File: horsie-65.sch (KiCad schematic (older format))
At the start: 17 parts, among them J1 AVR-ISP-6, J2 Connector_Generic_Conn_01x04, SW68 SW_Push, U2 ATmega32U4-AU, Y1 Crystal_GND24_Small

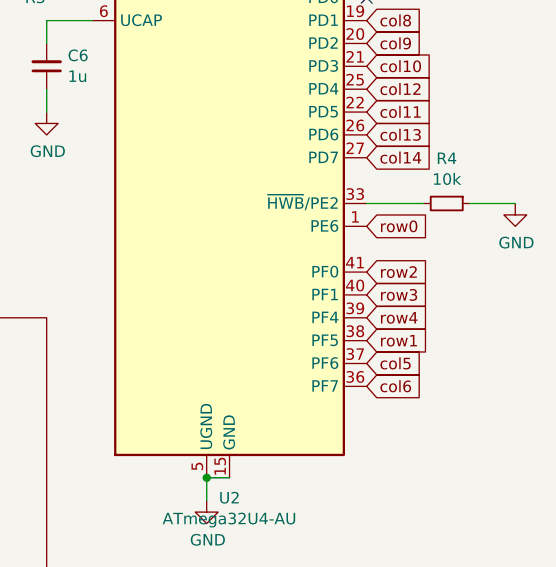
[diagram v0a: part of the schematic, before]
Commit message: more routing
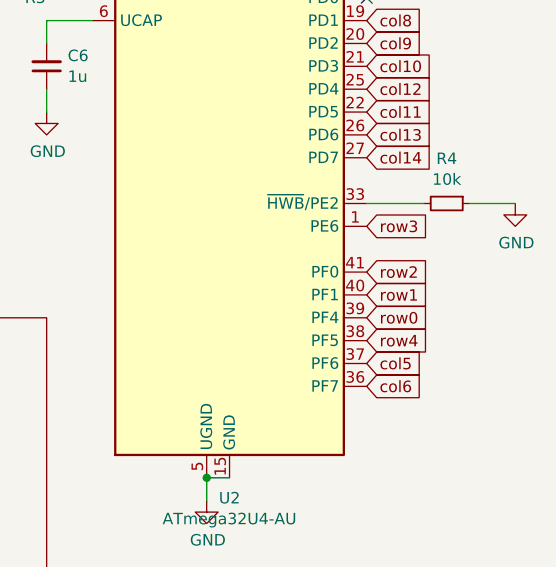
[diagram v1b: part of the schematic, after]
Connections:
- net row0: now also U2.39 (PF4); no longer U2.1 (PE6)
- net row1: now also U2.40 (PF1); no longer U2.38 (PF5)
- net row3: now also U2.1 (PE6); no longer U2.40 (PF1)
- net row4: now also U2.38 (PF5); no longer U2.39 (PF4)
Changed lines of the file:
@@
 Text GLabel 6900 3750 2    50   Input ~ 0
 col14
-Text GLabel 6900 4050 2    50   Input ~ 0
+Text GLabel 6900 4450 2    50   Input ~ 0
 row0
 Text GLabel 6900 4250 2    50   Input ~ 0
 row2
+Text GLabel 6900 4050 2    50   Input ~ 0
+row3
+Text GLabel 6900 4550 2    50   Input ~ 0
+row4
 Text GLabel 6900 4350 2    50   Input ~ 0
-row3
-Text GLabel 6900 4450 2    50   Input ~ 0
-row4
-Text GLabel 6900 4550 2    50   Input ~ 0
 row1
 Text GLabel 6900 4650 2    50   Input ~ 0
@@
 	3000 1600 3350 1600
 $Comp
-L power:+5V #PWR?
+L power:+5V #PWR0101
 U 1 1 63005D74
 P 3150 2600
-F 0 "#PWR?" H 3150 2450 50  0001 C CNN
+F 0 "#PWR0101" H 3150 2450 50  0001 C CNN
 F 1 "+5V" H 3165 2773 50  0000 C CNN
 F 2 "" H 3150 2600 50  0001 C CNN

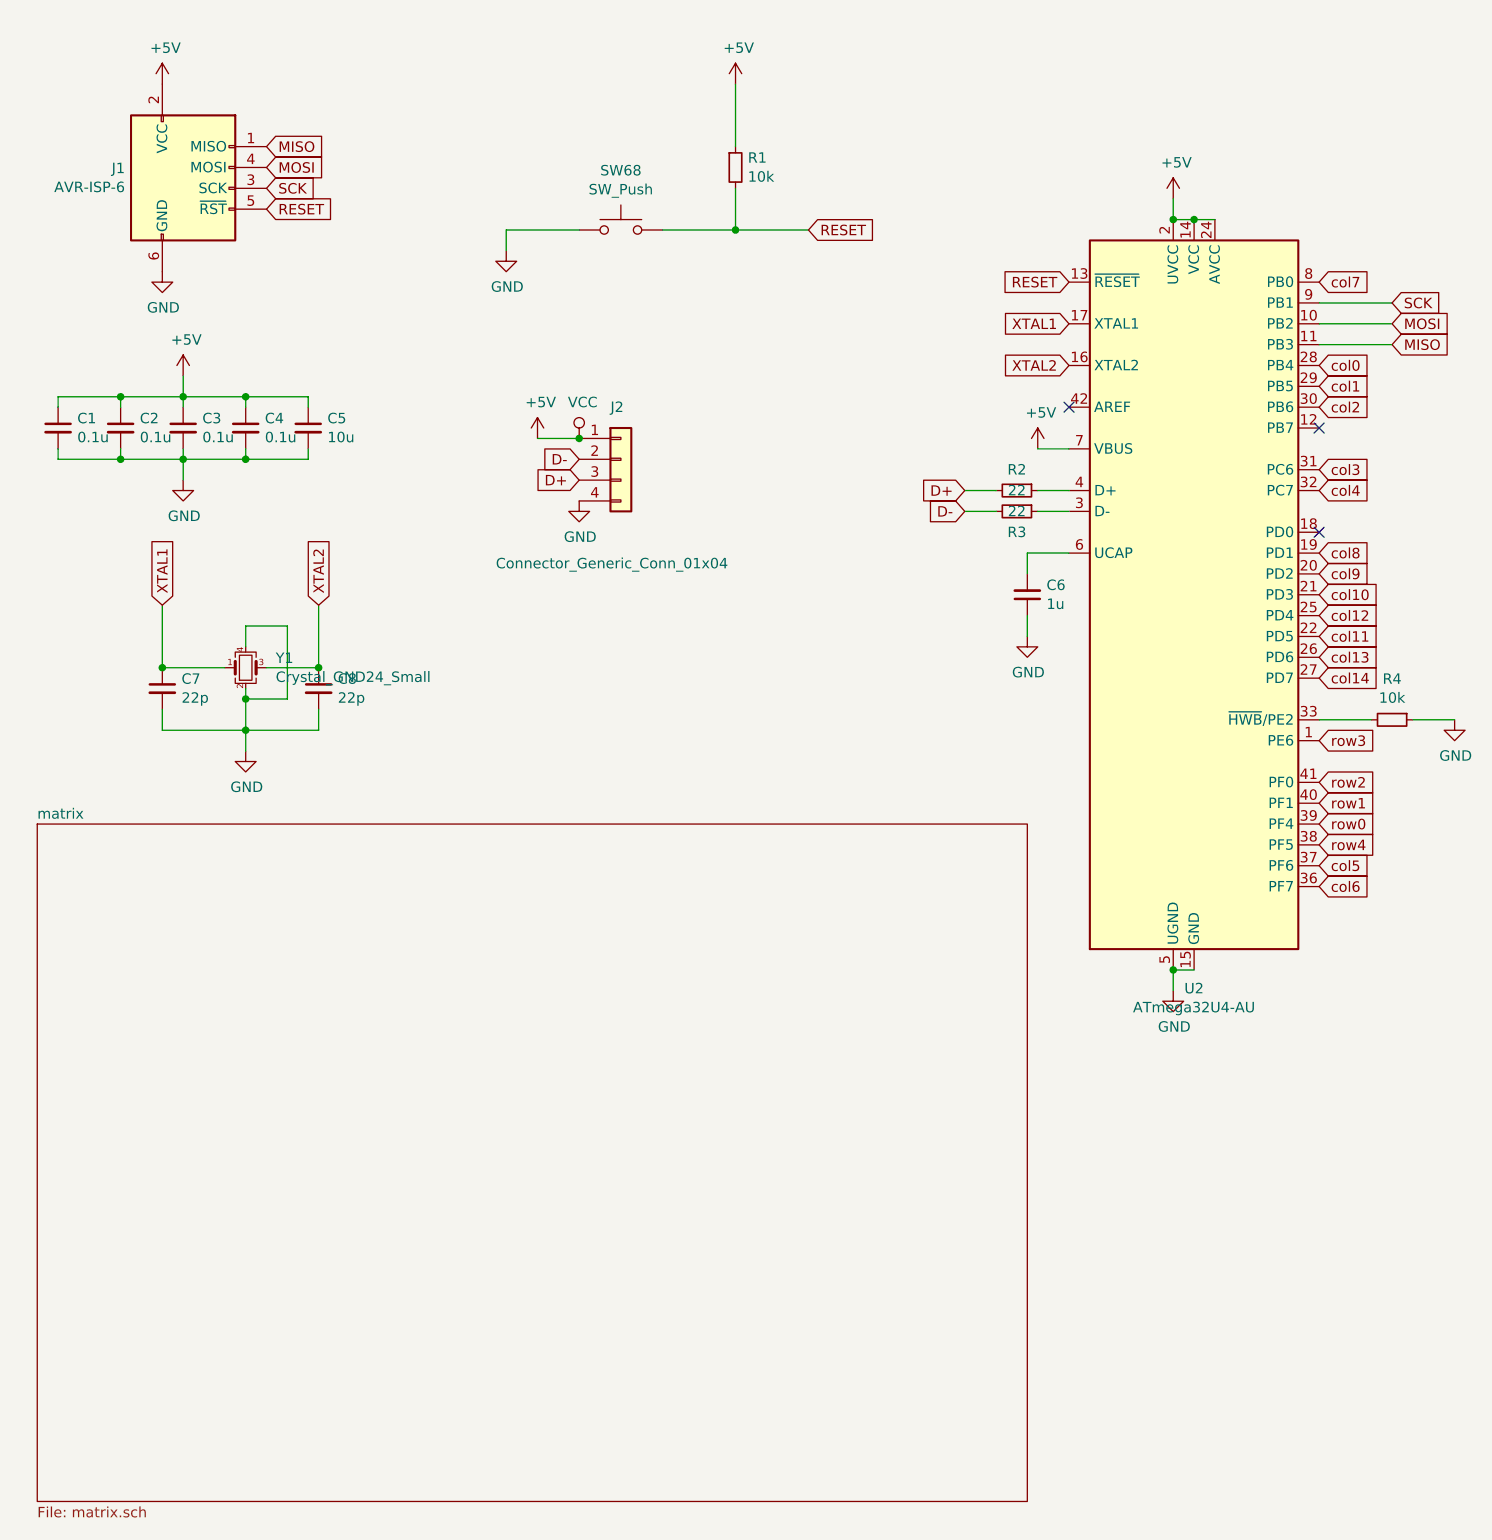
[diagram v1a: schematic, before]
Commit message: aesthetics 1
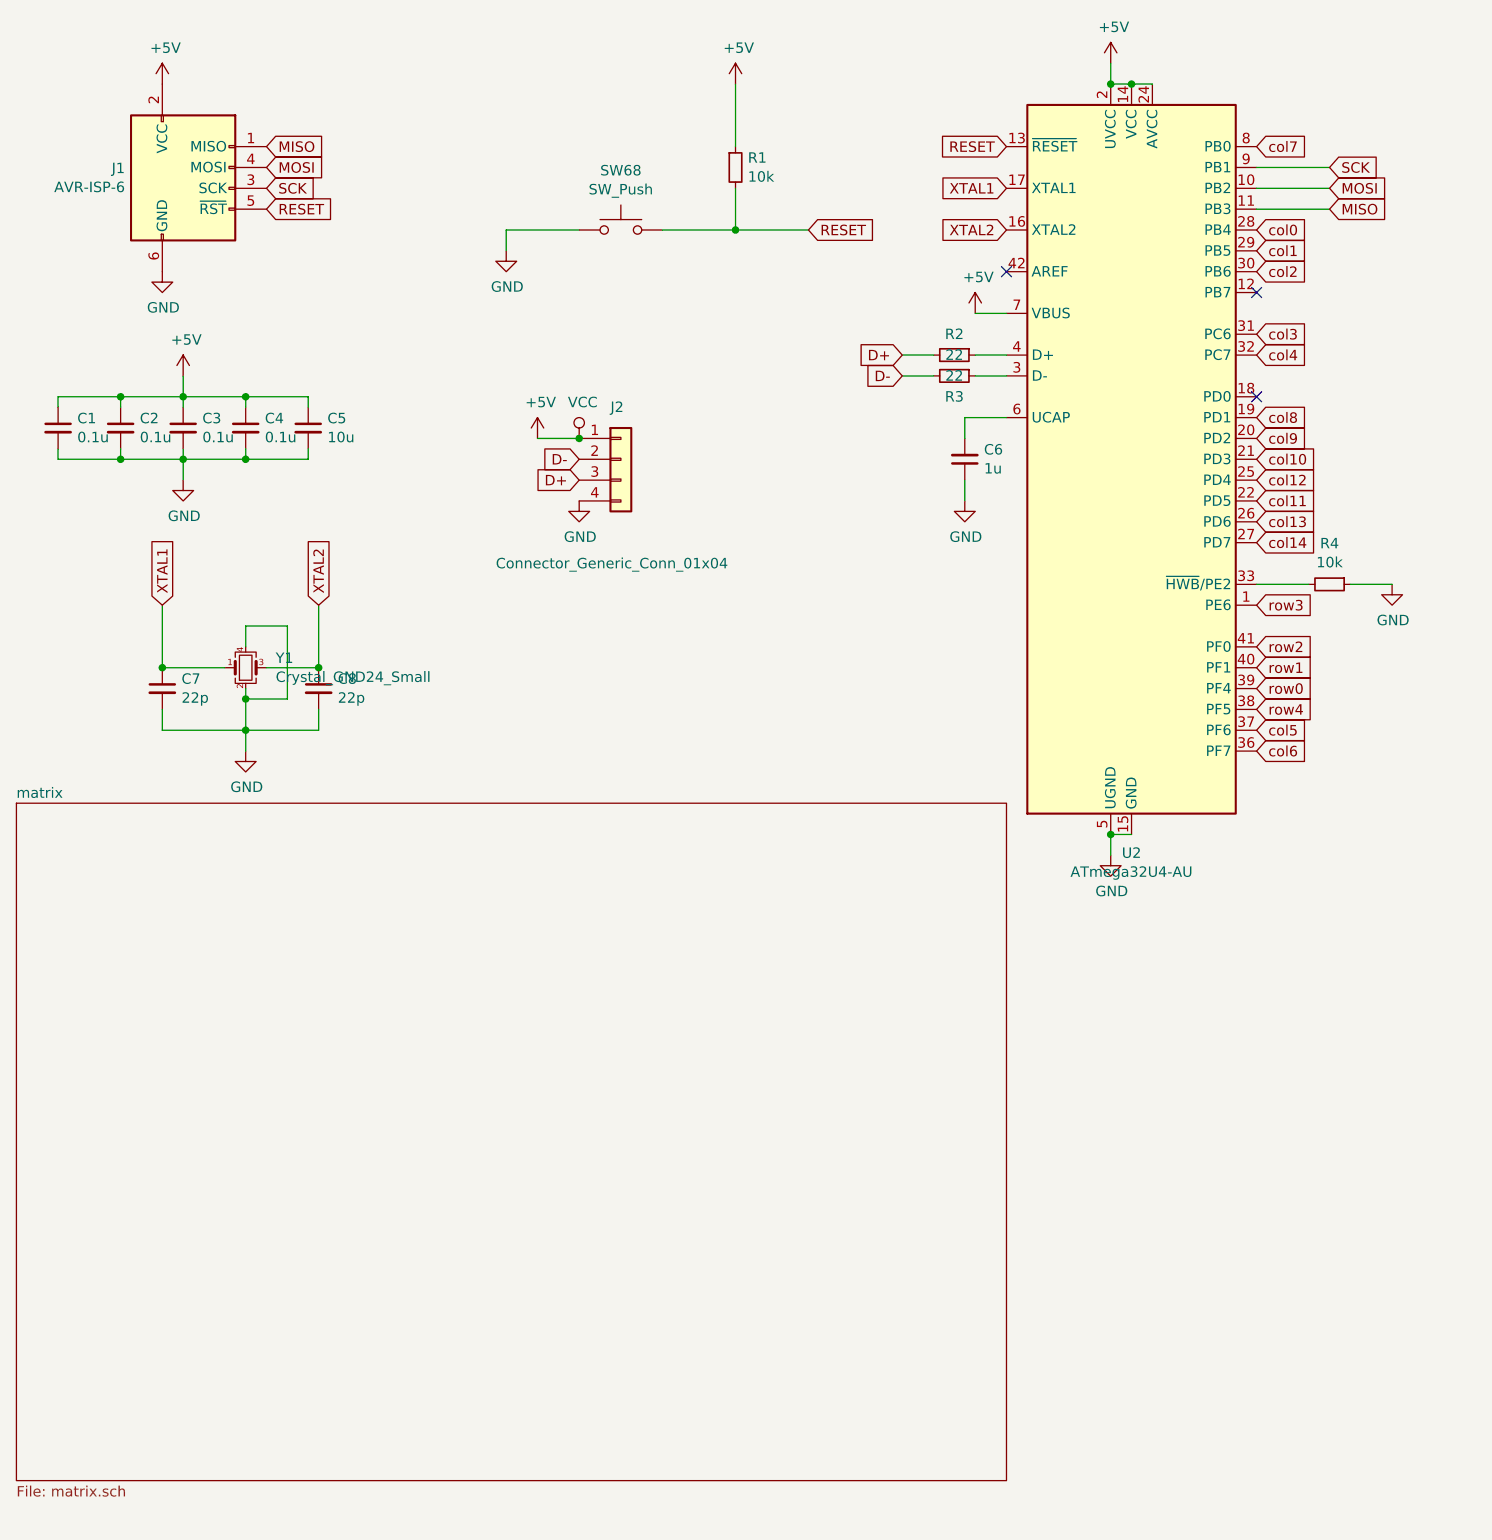
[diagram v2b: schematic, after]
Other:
- moved on the sheet: C6, R2, R3, R4, U2
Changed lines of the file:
@@
 L MCU_Microchip_ATmega:ATmega32U4-AU U2
 U 1 1 6283C2E5
-P 6300 3350
-F 0 "U2" H 6300 1461 50  0000 C CNN
-F 1 "ATmega32U4-AU" H 6300 1370 50  0000 C CNN
-F 2 "Package_QFP:TQFP-44_10x10mm_P0.8mm" H 6300 3350 50  0001 C CIN
-F 3 "http://ww1.microchip.com/downloads/en/DeviceDoc/Atmel-7766-8-bit-AVR-ATmega16U4-32U4_Datasheet.pdf" H 6300 3350 50  0001 C CNN
-	1    6300 3350
+P 6000 2700
+F 0 "U2" H 6000 811 50  0000 C CNN
+F 1 "ATmega32U4-AU" H 6000 720 50  0000 C CNN
+F 2 "Package_QFP:TQFP-44_10x10mm_P0.8mm" H 6000 2700 50  0001 C CIN
+F 3 "http://ww1.microchip.com/downloads/en/DeviceDoc/Atmel-7766-8-bit-AVR-ATmega16U4-32U4_Datasheet.pdf" H 6000 2700 50  0001 C CNN
+	1    6000 2700
 	1    0    0    -1
 $EndComp
@@
 L power:+5V #PWR03
 U 1 1 6283F3B3
-P 6200 1450
-F 0 "#PWR03" H 6200 1300 50  0001 C CNN
-F 1 "+5V" H 6215 1623 50  0000 C CNN
-F 2 "" H 6200 1450 50  0001 C CNN
-F 3 "" H 6200 1450 50  0001 C CNN
-	1    6200 1450
-	1    0    0    -1
-$EndComp
-Wire Wire Line
-	6200 1450 6200 1550
-Wire Wire Line
-	6200 1550 6300 1550
-Connection ~ 6200 1550
-Wire Wire Line
-	6300 1550 6400 1550
-Connection ~ 6300 1550
-Wire Wire Line
-	6300 5150 6200 5150
+P 5900 800
+F 0 "#PWR03" H 5900 650 50  0001 C CNN
+F 1 "+5V" H 5915 973 50  0000 C CNN
+F 2 "" H 5900 800 50  0001 C CNN
+F 3 "" H 5900 800 50  0001 C CNN
+	1    5900 800
+	1    0    0    -1
+$EndComp
+Wire Wire Line
+	5900 800  5900 900
+Wire Wire Line
+	5900 900  6000 900
+Connection ~ 5900 900
+Wire Wire Line
+	6000 900  6100 900
+Connection ~ 6000 900
+Wire Wire Line
+	6000 4500 5900 4500
 $Comp
 L power:GND #PWR014
 U 1 1 6284044C
-P 6200 5250
-F 0 "#PWR014" H 6200 5000 50  0001 C CNN
-F 1 "GND" H 6205 5077 50  0000 C CNN
-F 2 "" H 6200 5250 50  0001 C CNN
-F 3 "" H 6200 5250 50  0001 C CNN
-	1    6200 5250
-	1    0    0    -1
-$EndComp
-Wire Wire Line
-	6200 5150 6200 5250
-Connection ~ 6200 5150
-Text GLabel 5700 2050 0    50   Input ~ 0
+P 5900 4600
+F 0 "#PWR014" H 5900 4350 50  0001 C CNN
+F 1 "GND" H 5905 4427 50  0000 C CNN
+F 2 "" H 5900 4600 50  0001 C CNN
+F 3 "" H 5900 4600 50  0001 C CNN
+	1    5900 4600
+	1    0    0    -1
+$EndComp
+Wire Wire Line
+	5900 4500 5900 4600
+Connection ~ 5900 4500
+Text GLabel 5400 1400 0    50   Input ~ 0
 XTAL1
-Text GLabel 5700 2250 0    50   Input ~ 0
+Text GLabel 5400 1600 0    50   Input ~ 0
 XTAL2
-Text GLabel 5200 2850 0    50   Input ~ 0
+Text GLabel 4900 2200 0    50   Input ~ 0
 D+
-Text GLabel 5200 2950 0    50   Input ~ 0
+Text GLabel 4900 2300 0    50   Input ~ 0
 D-
 $Comp
 L Device:R_Small R4
 U 1 1 62841E9C
-P 7250 3950
-F 0 "R4" V 7054 3950 50  0000 C CNN
-F 1 "10k" V 7145 3950 50  0000 C CNN
-F 2 "Resistor_SMD:R_0805_2012Metric_Pad1.15x1.40mm_HandSolder" H 7250 3950 50  0001 C CNN
-F 3 "~" H 7250 3950 50  0001 C CNN
-	1    7250 3950
+P 6950 3300
+F 0 "R4" V 6754 3300 50  0000 C CNN
+F 1 "10k" V 6845 3300 50  0000 C CNN
+F 2 "Resistor_SMD:R_0805_2012Metric_Pad1.15x1.40mm_HandSolder" H 6950 3300 50  0001 C CNN
+F 3 "~" H 6950 3300 50  0001 C CNN
+	1    6950 3300
 	0    1    1    0
 $EndComp
 Wire Wire Line
-	6900 3950 7150 3950
+	6600 3300 6850 3300
 $Comp
 L power:GND #PWR012
 U 1 1 62843533
-P 7550 3950
-F 0 "#PWR012" H 7550 3700 50  0001 C CNN
-F 1 "GND" H 7555 3777 50  0000 C CNN
-F 2 "" H 7550 3950 50  0001 C CNN
-F 3 "" H 7550 3950 50  0001 C CNN
-	1    7550 3950
-	1    0    0    -1
-$EndComp
-Wire Wire Line
-	7550 3950 7350 3950
-NoConn ~ 5700 2450
+P 7250 3300
+F 0 "#PWR012" H 7250 3050 50  0001 C CNN
+F 1 "GND" H 7255 3127 50  0000 C CNN
+F 2 "" H 7250 3300 50  0001 C CNN
+F 3 "" H 7250 3300 50  0001 C CNN
+	1    7250 3300
+	1    0    0    -1
+$EndComp
+Wire Wire Line
+	7250 3300 7050 3300
+NoConn ~ 5400 1800
 $Comp
 L power:+5V #PWR08
 U 1 1 62844DBF
-P 5550 2650
-F 0 "#PWR08" H 5550 2500 50  0001 C CNN
-F 1 "+5V" H 5565 2823 50  0000 C CNN
-F 2 "" H 5550 2650 50  0001 C CNN
-F 3 "" H 5550 2650 50  0001 C CNN
-	1    5550 2650
-	1    0    0    -1
-$EndComp
-Wire Wire Line
-	5550 2650 5700 2650
-Text GLabel 5700 1850 0    50   Input ~ 0
+P 5250 2000
+F 0 "#PWR08" H 5250 1850 50  0001 C CNN
+F 1 "+5V" H 5265 2173 50  0000 C CNN
+F 2 "" H 5250 2000 50  0001 C CNN
+F 3 "" H 5250 2000 50  0001 C CNN
+	1    5250 2000
+	1    0    0    -1
+$EndComp
+Wire Wire Line
+	5250 2000 5400 2000
+Text GLabel 5400 1200 0    50   Input ~ 0
 RESET
-Text GLabel 7250 1950 2    50   Input ~ 0
+Text GLabel 6950 1300 2    50   Input ~ 0
 SCK
-Text GLabel 7250 2050 2    50   Input ~ 0
+Text GLabel 6950 1400 2    50   Input ~ 0
 MOSI
-Text GLabel 7250 2150 2    50   Input ~ 0
+Text GLabel 6950 1500 2    50   Input ~ 0
 MISO
 Wire Wire Line
-	7250 2050 6900 2050
-Wire Wire Line
-	6900 1950 7250 1950
+	6950 1400 6600 1400
+Wire Wire Line
+	6600 1300 6950 1300
 $Comp
 L Device:C_Small C6
 U 1 1 62846732
-P 5500 3350
-F 0 "C6" H 5408 3304 50  0000 R CNN
-F 1 "1u" H 5408 3395 50  0000 R CNN
-F 2 "Capacitor_SMD:C_0805_2012Metric_Pad1.15x1.40mm_HandSolder" H 5500 3350 50  0001 C CNN
-F 3 "~" H 5500 3350 50  0001 C CNN
-	1    5500 3350
+P 5200 2700
+F 0 "C6" H 5108 2654 50  0000 R CNN
+F 1 "1u" H 5108 2745 50  0000 R CNN
+F 2 "Capacitor_SMD:C_0805_2012Metric_Pad1.15x1.40mm_HandSolder" H 5200 2700 50  0001 C CNN
+F 3 "~" H 5200 2700 50  0001 C CNN
+	1    5200 2700
 	-1   0    0    1
 $EndComp
 Wire Wire Line
-	5700 3150 5500 3150
-Wire Wire Line
-	5500 3150 5500 3250
+	5400 2500 5200 2500
+Wire Wire Line
+	5200 2500 5200 2600
 $Comp
 L power:GND #PWR011
 U 1 1 62847E4C
-P 5500 3550
-F 0 "#PWR011" H 5500 3300 50  0001 C CNN
-F 1 "GND" H 5505 3377 50  0000 C CNN
-F 2 "" H 5500 3550 50  0001 C CNN
-F 3 "" H 5500 3550 50  0001 C CNN
-	1    5500 3550
-	1    0    0    -1
-$EndComp
-Wire Wire Line
-	5500 3550 5500 3450
-Wire Wire Line
-	6900 2150 7250 2150
+P 5200 2900
+F 0 "#PWR011" H 5200 2650 50  0001 C CNN
+F 1 "GND" H 5205 2727 50  0000 C CNN
+F 2 "" H 5200 2900 50  0001 C CNN
+F 3 "" H 5200 2900 50  0001 C CNN
+	1    5200 2900
+	1    0    0    -1
+$EndComp
+Wire Wire Line
+	5200 2900 5200 2800
+Wire Wire Line
+	6600 1500 6950 1500
 Text GLabel 4450 1600 2    50   Input ~ 0
 RESET
@@
 L Device:R_Small R2
 U 1 1 62881754
-P 5450 2850
-F 0 "R2" V 5350 2850 50  0000 C CNN
-F 1 "22" V 5450 2850 50  0000 C CNN
-F 2 "Resistor_SMD:R_0805_2012Metric_Pad1.15x1.40mm_HandSolder" H 5450 2850 50  0001 C CNN
-F 3 "~" H 5450 2850 50  0001 C CNN
-	1    5450 2850
+P 5150 2200
+F 0 "R2" V 5050 2200 50  0000 C CNN
+F 1 "22" V 5150 2200 50  0000 C CNN
+F 2 "Resistor_SMD:R_0805_2012Metric_Pad1.15x1.40mm_HandSolder" H 5150 2200 50  0001 C CNN
+F 3 "~" H 5150 2200 50  0001 C CNN
+	1    5150 2200
 	0    1    1    0
 $EndComp
@@
 L Device:R_Small R3
 U 1 1 62881CC4
-P 5450 2950
-F 0 "R3" V 5550 2950 50  0000 C CNN
-F 1 "22" V 5450 2950 50  0000 C CNN
-F 2 "Resistor_SMD:R_0805_2012Metric_Pad1.15x1.40mm_HandSolder" H 5450 2950 50  0001 C CNN
-F 3 "~" H 5450 2950 50  0001 C CNN
-	1    5450 2950
+P 5150 2300
+F 0 "R3" V 5250 2300 50  0000 C CNN
+F 1 "22" V 5150 2300 50  0000 C CNN
+F 2 "Resistor_SMD:R_0805_2012Metric_Pad1.15x1.40mm_HandSolder" H 5150 2300 50  0001 C CNN
+F 3 "~" H 5150 2300 50  0001 C CNN
+	1    5150 2300
 	0    1    1    0
 $EndComp
 Wire Wire Line
-	5350 2850 5200 2850
-Wire Wire Line
-	5200 2950 5350 2950
-Wire Wire Line
-	5550 2950 5700 2950
-Wire Wire Line
-	5700 2850 5550 2850
+	5050 2200 4900 2200
+Wire Wire Line
+	4900 2300 5050 2300
+Wire Wire Line
+	5250 2300 5400 2300
+Wire Wire Line
+	5400 2200 5250 2200
 $Comp
 L Connector:AVR-ISP-6 J1
@@
 Wire Wire Line
 	1750 3850 1750 4000
-$Sheet
-S 750  4450 4750 3250
-U 628A0341
-F0 "matrix" 50
-F1 "matrix.sch" 50
-$EndSheet
-Text GLabel 6900 1850 2    50   Input ~ 0
+Text GLabel 6600 1200 2    50   Input ~ 0
 col7
-Text GLabel 6900 2250 2    50   Input ~ 0
+Text GLabel 6600 1600 2    50   Input ~ 0
 col0
-Text GLabel 6900 2350 2    50   Input ~ 0
+Text GLabel 6600 1700 2    50   Input ~ 0
 col1
-Text GLabel 6900 2450 2    50   Input ~ 0
+Text GLabel 6600 1800 2    50   Input ~ 0
 col2
-NoConn ~ 6900 2550
-Text GLabel 6900 2750 2    50   Input ~ 0
+NoConn ~ 6600 1900
+Text GLabel 6600 2100 2    50   Input ~ 0
 col3
-Text GLabel 6900 2850 2    50   Input ~ 0
+Text GLabel 6600 2200 2    50   Input ~ 0
 col4
-NoConn ~ 6900 3050
-Text GLabel 6900 3150 2    50   Input ~ 0
+NoConn ~ 6600 2400
+Text GLabel 6600 2500 2    50   Input ~ 0
 col8
-Text GLabel 6900 3250 2    50   Input ~ 0
+Text GLabel 6600 2600 2    50   Input ~ 0
 col9
-Text GLabel 6900 3350 2    50   Input ~ 0
+Text GLabel 6600 2700 2    50   Input ~ 0
 col10
-Text GLabel 6900 3450 2    50   Input ~ 0
+Text GLabel 6600 2800 2    50   Input ~ 0
 col12
-Text GLabel 6900 3550 2    50   Input ~ 0
+Text GLabel 6600 2900 2    50   Input ~ 0
 col11
-Text GLabel 6900 3650 2    50   Input ~ 0
+Text GLabel 6600 3000 2    50   Input ~ 0
 col13
-Text GLabel 6900 3750 2    50   Input ~ 0
+Text GLabel 6600 3100 2    50   Input ~ 0
 col14
-Text GLabel 6900 4450 2    50   Input ~ 0
+Text GLabel 6600 3800 2    50   Input ~ 0
 row0
-Text GLabel 6900 4250 2    50   Input ~ 0
+Text GLabel 6600 3600 2    50   Input ~ 0
 row2
-Text GLabel 6900 4050 2    50   Input ~ 0
+Text GLabel 6600 3400 2    50   Input ~ 0
 row3
-Text GLabel 6900 4550 2    50   Input ~ 0
+Text GLabel 6600 3900 2    50   Input ~ 0
 row4
-Text GLabel 6900 4350 2    50   Input ~ 0
+Text GLabel 6600 3700 2    50   Input ~ 0
 row1
-Text GLabel 6900 4650 2    50   Input ~ 0
+Text GLabel 6600 4000 2    50   Input ~ 0
 col5
-Text GLabel 6900 4750 2    50   Input ~ 0
+Text GLabel 6600 4100 2    50   Input ~ 0
 col6
 $Comp
@@
 	3150 2600 3350 2600
 Connection ~ 3350 2600
+$Sheet
+S 650  4350 4750 3250
+U 628A0341
+F0 "matrix" 50
+F1 "matrix.sch" 50
+$EndSheet
 $EndSCHEMATC
